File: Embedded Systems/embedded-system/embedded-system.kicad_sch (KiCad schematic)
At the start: 9 parts, among them M1 Motor_Servo, M2 Motor_Servo

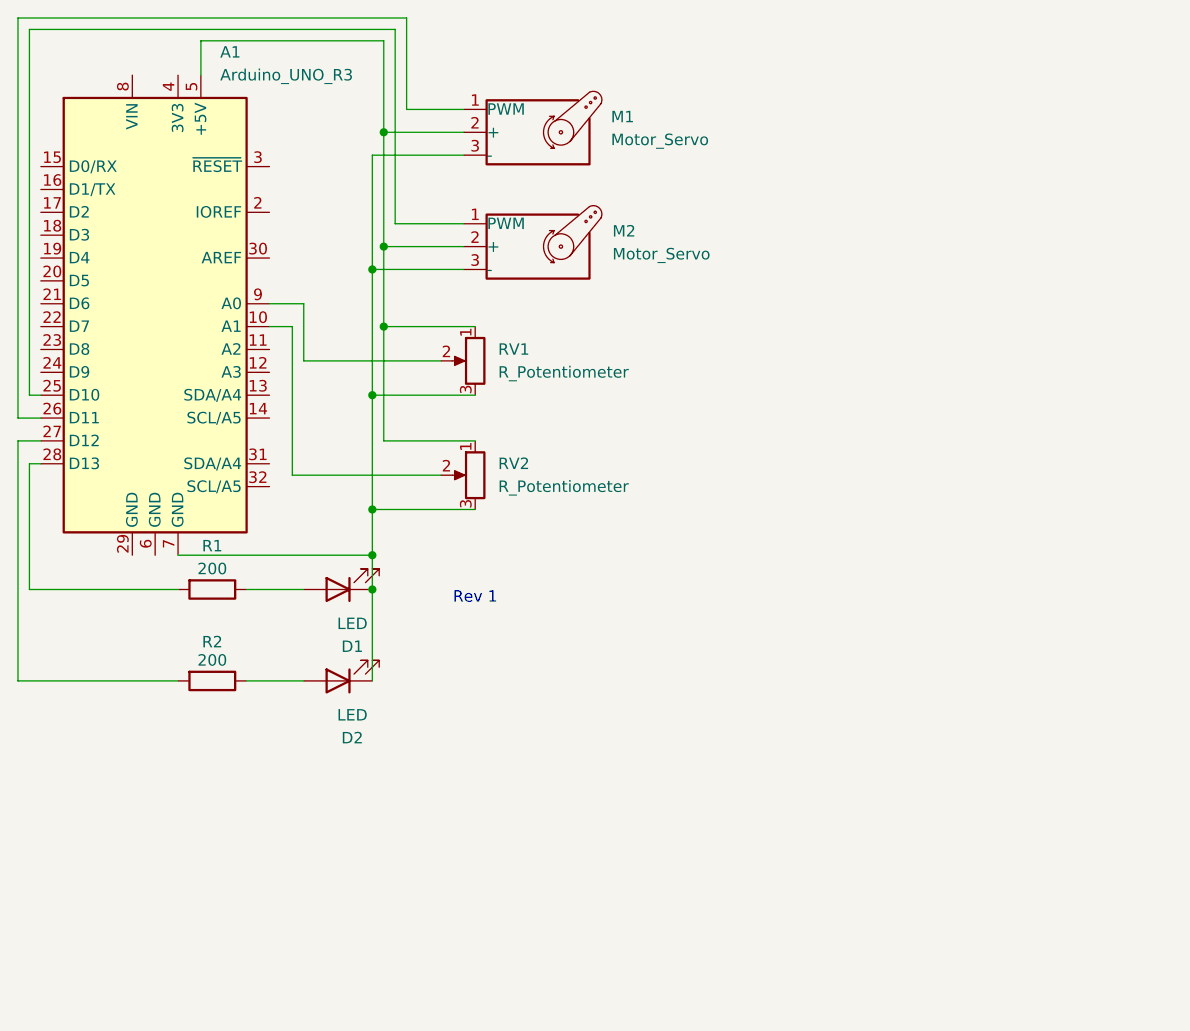
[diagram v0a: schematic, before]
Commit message: feat: updated schematic
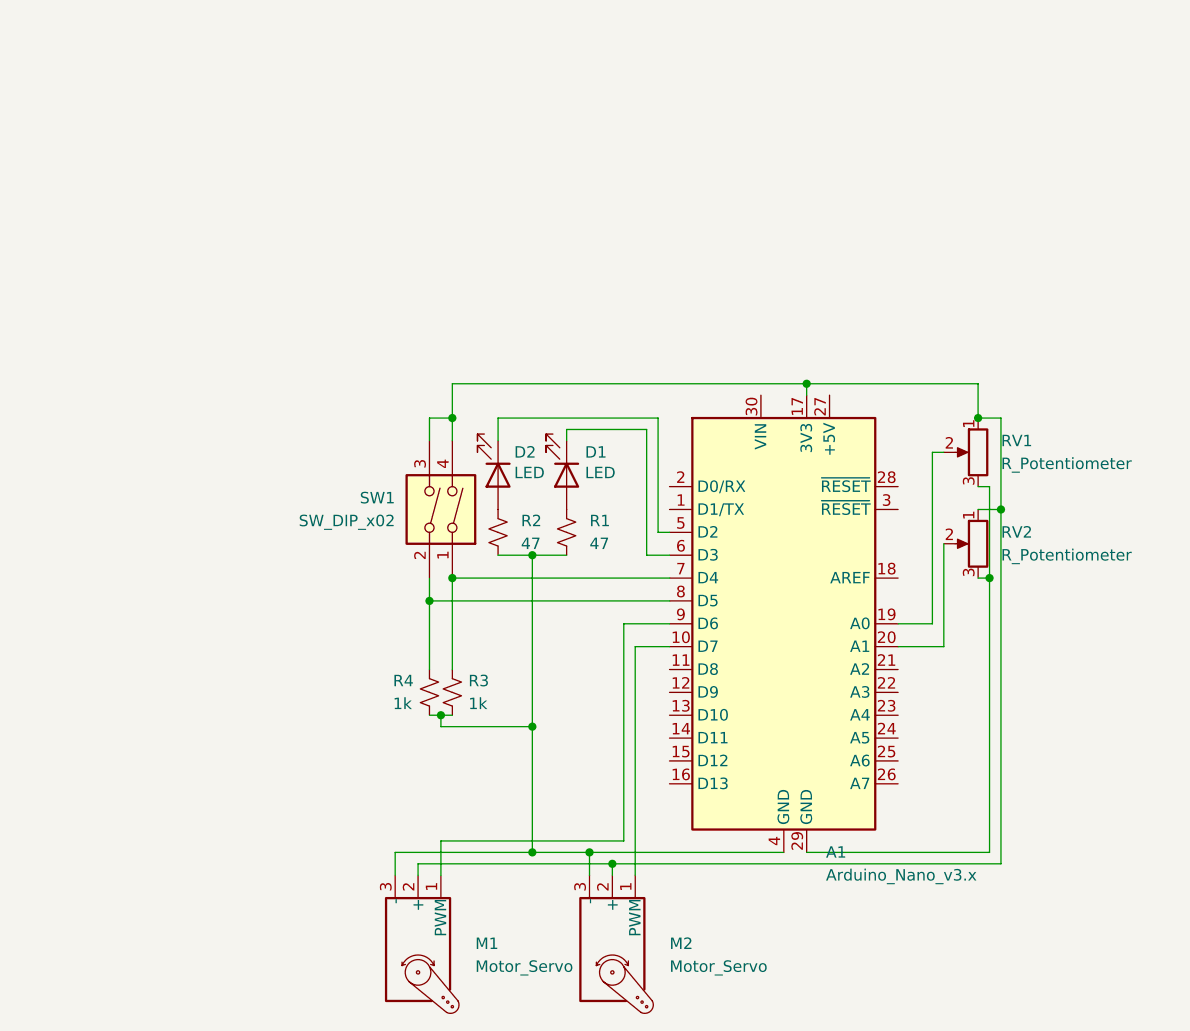
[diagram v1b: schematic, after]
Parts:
- removed A1: Arduino_UNO_R3, Module:Arduino_UNO_R3, symbol MCU_Module:Arduino_UNO_R3
- removed R1, R2: 200, symbol Device:R
- added A1: Arduino_Nano_v3.x, Module:Arduino_Nano, symbol MCU_Module:Arduino_Nano_v3.x
- added R1, R2: 47, Resistor_THT:R_Axial_DIN0207_L6.3mm_D2.5mm_P10.16mm_Horizontal, symbol Device:R_Small_US
- added R3, R4: 1k, Resistor_THT:R_Axial_DIN0207_L6.3mm_D2.5mm_P10.16mm_Horizontal, symbol Device:R_Small_US
- added SW1: SW_DIP_x02, Button_Switch_THT:SW_DIP_SPSTx02_Piano_10.8x6.64mm_W7.62mm_P2.54mm, symbol Switch:SW_DIP_x02
- D1, D2: footprint LED_THT:LED_D5.0mm_Horizontal_O6.35mm_Z15.0mm -> LED_THT:LED_D5.0mm
- RV1, RV2: footprint custom-footprint:p103 -> Potentiometer_THT:Potentiometer_ACP_CA14-H5_Horizontal
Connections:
- net at D1.2 (A): now also R1.1
- net at M1.2 (+), M2.2 (+), RV1.1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: now also A1.17 (3V3), SW1.3, SW1.4
- net at RV1.2: now also A1.19 (A0)
- net at M2.1 (PWM): now also A1.10 (D7)
- net at M1.1 (PWM): now also A1.9 (D6)
- net at RV2.2: now also A1.20 (A1)
- net at D2.2 (A): now also R2.1
- new net: A1.4 (GND), M1.3 (-), M2.3 (-), R1.2, R2.2, R3.2, R4.2
- new net: A1.29 (GND), RV1.3, RV2.3
- new net: A1.5 (D2), D2.1 (K)
- new net: A1.6 (D3), D1.1 (K)
- new net: A1.7 (D4), R3.1, SW1.1
- new net: A1.8 (D5), R4.1, SW1.2
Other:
- note removed: "Rev 1"
